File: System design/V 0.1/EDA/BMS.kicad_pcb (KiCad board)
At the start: 2 copper layers, 26 x 70 mm, 20 parts, among them J1 Conn_01x03_Pin, J2 Conn_01x02_Pin, Q1 NMOS, Q2 NMOS, Q3 PMOS, Q4 PMOS, U1 SN74LVC2G14DBV, U2 SN74LVC2G14DBV, U3 CDSOT236-0504C

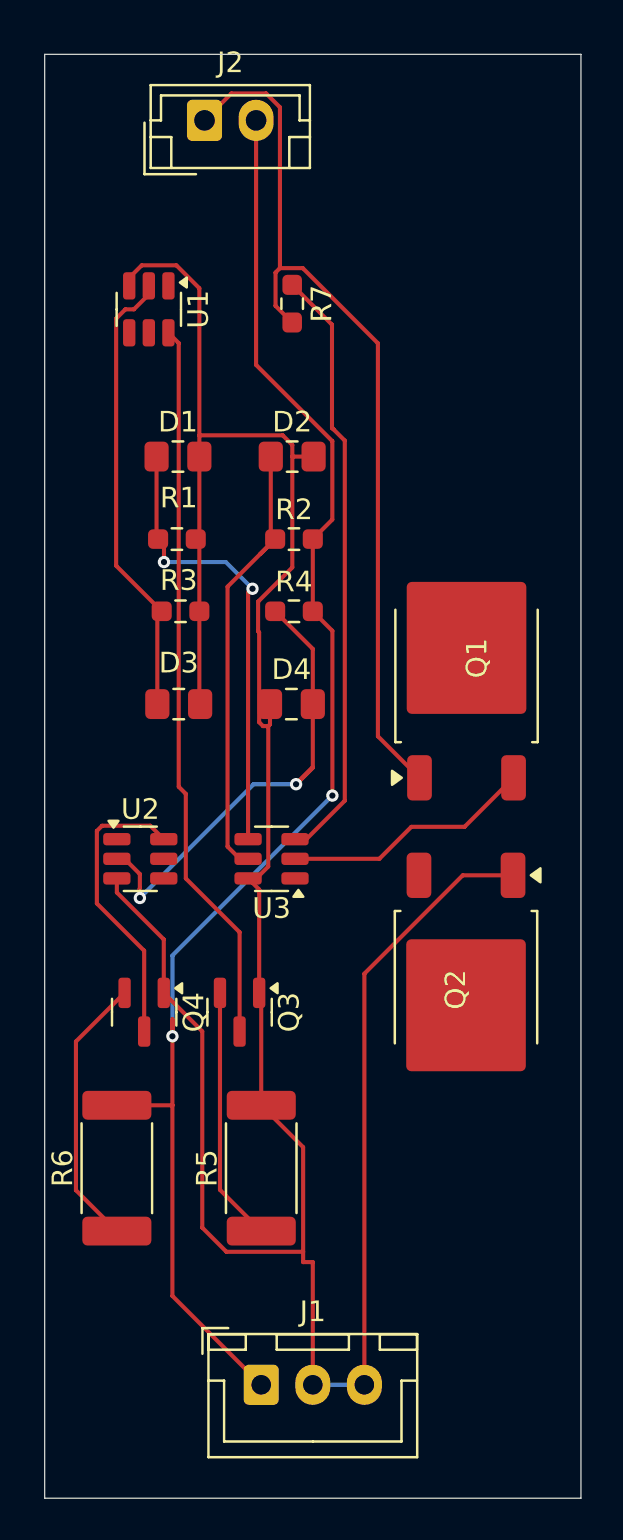
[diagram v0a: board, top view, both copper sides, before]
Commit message: Updated Directory
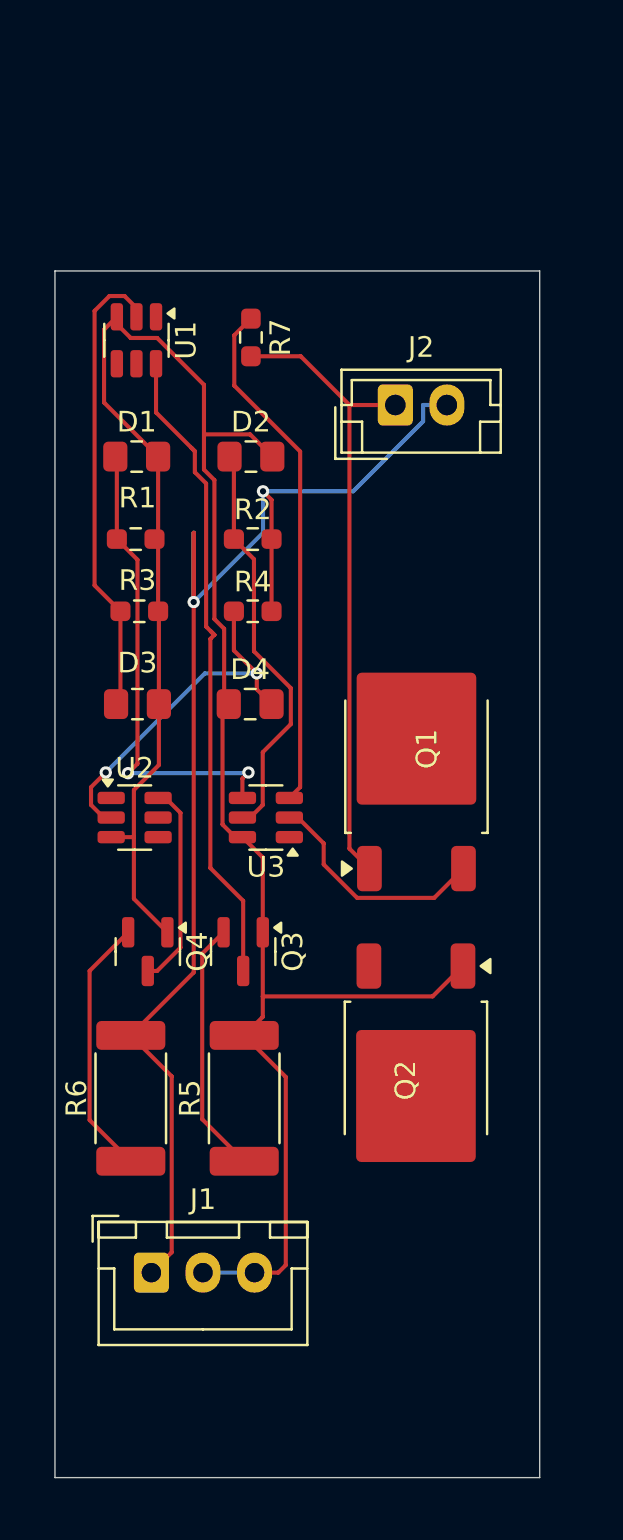
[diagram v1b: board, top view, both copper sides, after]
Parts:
- moved J2 16.6 mm to (151.5, 70.5)
- moved J1 7.61 mm to (139.7, 112.6)
- moved Q1 5.03 mm to (152.5, 87.9)
- moved Q2 5.03 mm to (152.5, 102.7)
- moved R5 3.49 mm to (144.2, 104.1)
- moved R6 3.45 mm to (138.7, 104.1)
- moved Q3 2.94 mm to (144.1, 97.0)
- moved Q4 2.94 mm to (139.5, 97.0)
- moved R7 2.58 mm to (144.5, 67.2)
- moved U3 2.02 mm to (145.2, 90.5)
- moved U2 2.02 mm to (138.9, 90.5)
- moved D1 2.00 mm to (139.0, 73.0)
- moved D2 2.00 mm to (144.5, 73.0)
- moved D3 2.00 mm to (139.0, 85.0)
- moved D4 2.00 mm to (144.5, 85.0)
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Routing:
- net Net-(D1-A): track 136.0 -> 103.1 mm
- net Net-(J2-Pin_1): track 43.5 -> 30.9 mm
- net Net-(D4-A): track 28.4 -> 17.7 mm
- net Net-(Q4-S): track 14.3 -> 9.97 mm
- net Net-(U3-IO2): track 29.4 -> 25.1 mm
- net Net-(Q3-S): track 35.3 -> 31.8 mm
- net Net-(J1-Pin_1): track 74.6 -> 72.3 mm
- net Net-(D2-K): track 22.0 -> 19.9 mm
- net Net-(Q1-S): track 12.2 -> 11.2 mm
- net Net-(Q4-G): track 13.3 -> 12.7 mm
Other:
- board size 26 x 70 mm -> 23.5 x 58.5 mm
